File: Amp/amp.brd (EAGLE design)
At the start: 97.8 x 53.3 mm, 45 parts, among them IC1 TL072P, Q1 BC550C, Q10 BC560, Q11 IRF520, Q12 IRF520, Q13 IRF520, Q2 BC560, Q3 BC560, Q4 BC550C, Q5 BC560, Q6 BC560, Q7 BC560, Q8 BC560, Q9 BC550C, U1 LM334Z, U2 TL431PTH, U3 LM334Z

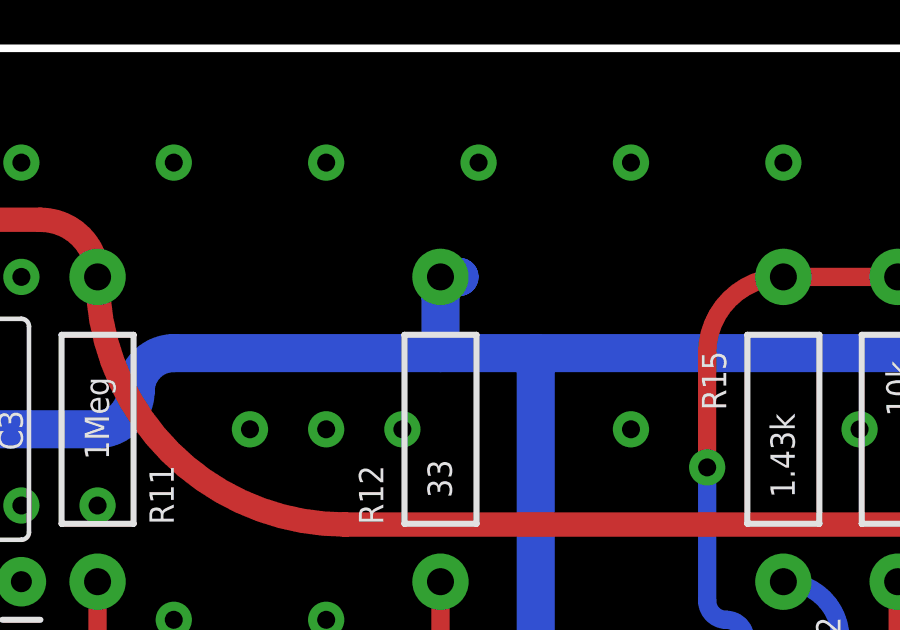
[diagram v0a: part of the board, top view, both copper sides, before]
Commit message: Oops
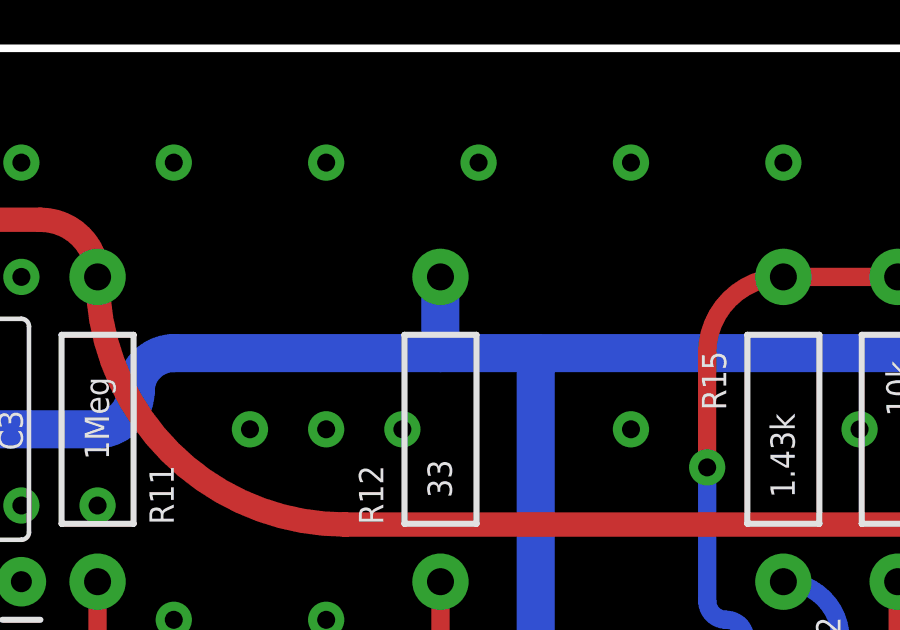
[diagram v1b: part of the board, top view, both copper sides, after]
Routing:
- net V+: track 189.0 -> 188.1 mm
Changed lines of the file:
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@@
 <wire x1="49.53" y1="17.78" x2="52.705" y2="20.955" width="1.27" layer="16" curve="90"/>
 <wire x1="52.705" y1="20.955" x2="52.705" y2="43.18" width="1.27" layer="16"/>
-<wire x1="50.165" y1="45.72" x2="49.53" y2="45.72" width="1.27" layer="16"/>
 <wire x1="52.705" y1="43.18" x2="67.31" y2="43.18" width="1.27" layer="16"/>
 <wire x1="67.31" y1="43.18" x2="87.63" y2="43.18" width="1.27" layer="16"/>
@@
 <wire x1="40.64" y1="43.18" x2="49.53" y2="43.18" width="1.27" layer="16"/>
 <wire x1="49.53" y1="43.18" x2="52.705" y2="43.18" width="1.27" layer="16"/>
-<wire x1="50.165" y1="45.72" x2="49.53" y2="45.085" width="1.27" layer="16" curve="90"/>
-<wire x1="49.53" y1="45.085" x2="49.53" y2="43.18" width="1.27" layer="16"/>
+<wire x1="49.53" y1="45.72" x2="49.53" y2="43.18" width="1.27" layer="16"/>
 </signal>
 <signal name="V-" class="1">
